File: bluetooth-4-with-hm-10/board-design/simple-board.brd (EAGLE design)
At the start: 20 x 31.7 mm, 5 parts

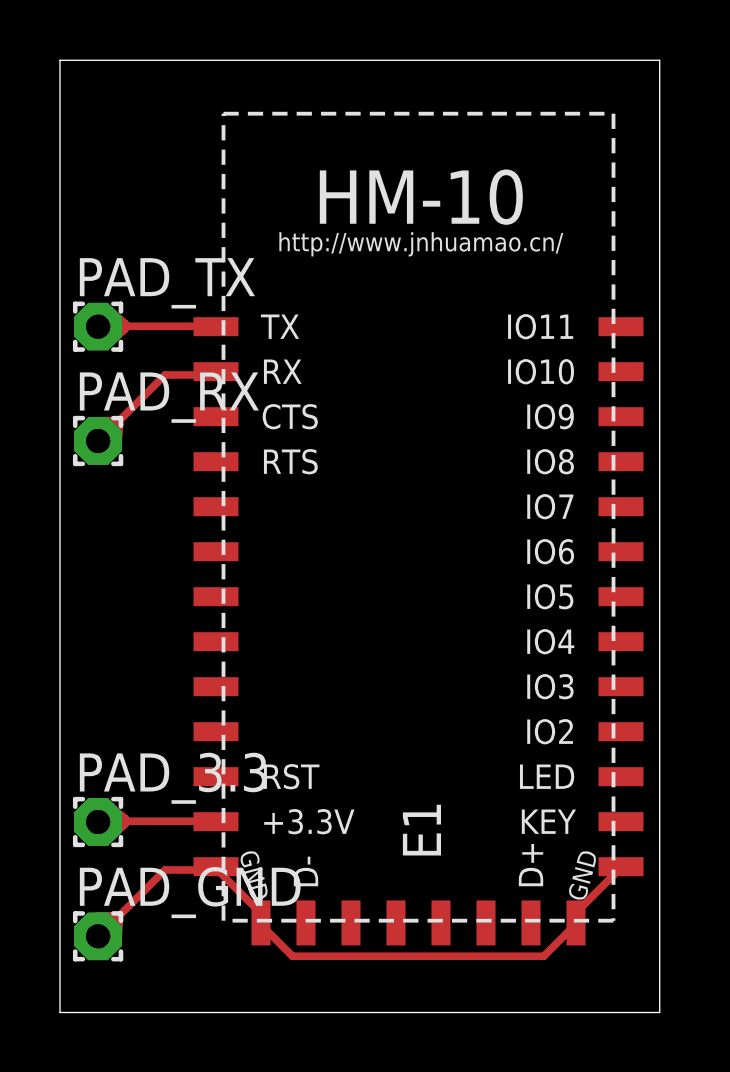
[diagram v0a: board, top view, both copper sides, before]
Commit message: Update: planeground board
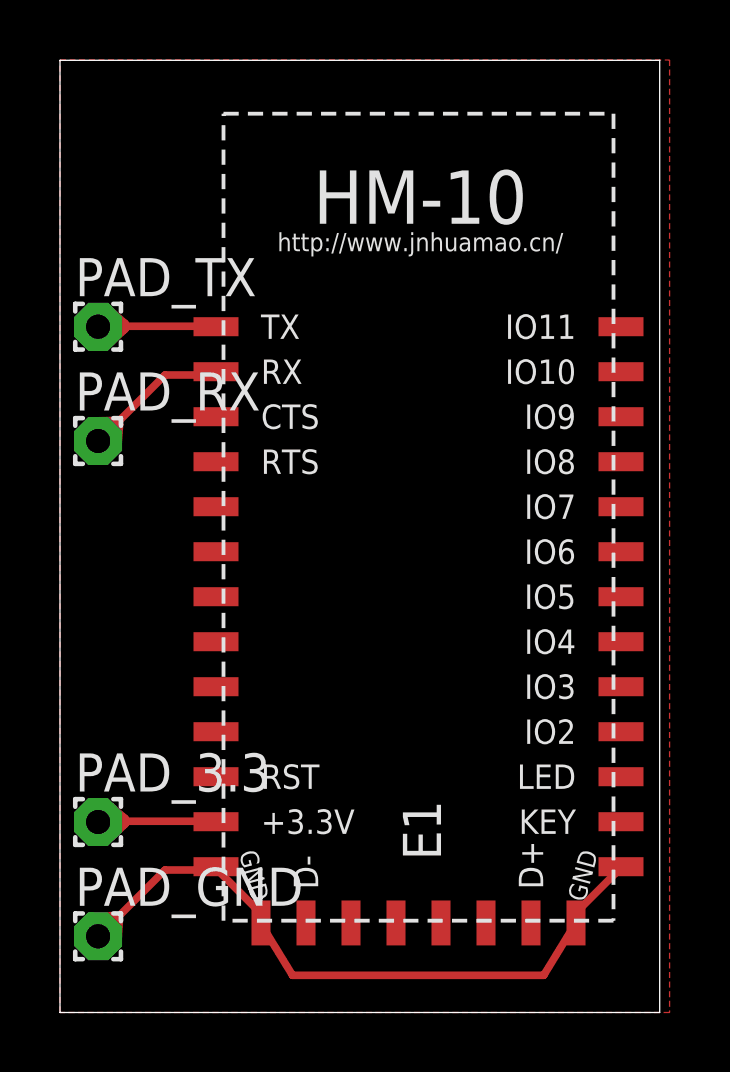
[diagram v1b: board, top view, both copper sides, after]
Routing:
- net GND: track 23.7 -> 24.7 mm
- added copper zone on layer 1, net N$1
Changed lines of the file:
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@@
 <wire x1="5.125" y1="4.75" x2="5.2" y2="4.86" width="0.254" layer="1"/>
 <wire x1="1.375" y1="2.625" x2="1.27" y2="2.54" width="0.254" layer="1"/>
-<wire x1="16.125" y1="1.875" x2="17.125" y2="2.875" width="0.254" layer="1"/>
-<wire x1="7.75" y1="1.875" x2="16.125" y2="1.875" width="0.254" layer="1"/>
-<wire x1="6.75" y1="2.875" x2="7.75" y2="1.875" width="0.254" layer="1"/>
+<wire x1="16.125" y1="1.24" x2="17.125" y2="2.875" width="0.254" layer="1"/>
+<wire x1="7.75" y1="1.24" x2="16.125" y2="1.24" width="0.254" layer="1"/>
+<wire x1="6.75" y1="2.875" x2="7.75" y2="1.24" width="0.254" layer="1"/>
 <wire x1="17.125" y1="2.875" x2="17.2" y2="2.985" width="0.254" layer="1"/>
 <wire x1="6.75" y1="2.875" x2="6.7" y2="2.985" width="0.254" layer="1"/>
@@
 <wire x1="1.27" y1="2.54" x2="1.814909375" y2="2.50395" width="0.508" layer="1"/>
 </signal>
+<signal name="N$1">
+<polygon width="0.5" layer="1" isolate="0.5">
+<vertex x="0" y="31.75"/>
+<vertex x="20.32" y="31.75"/>
+<vertex x="20.32" y="0"/>
+<vertex x="0" y="0"/>
+</polygon>
+</signal>
 </signals>
